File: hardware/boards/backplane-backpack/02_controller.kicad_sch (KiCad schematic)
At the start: 12 parts, among them J10 GND/+3V3/SWDIO/SWCLK/NRST (TB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, U1 STM32C092FCP6

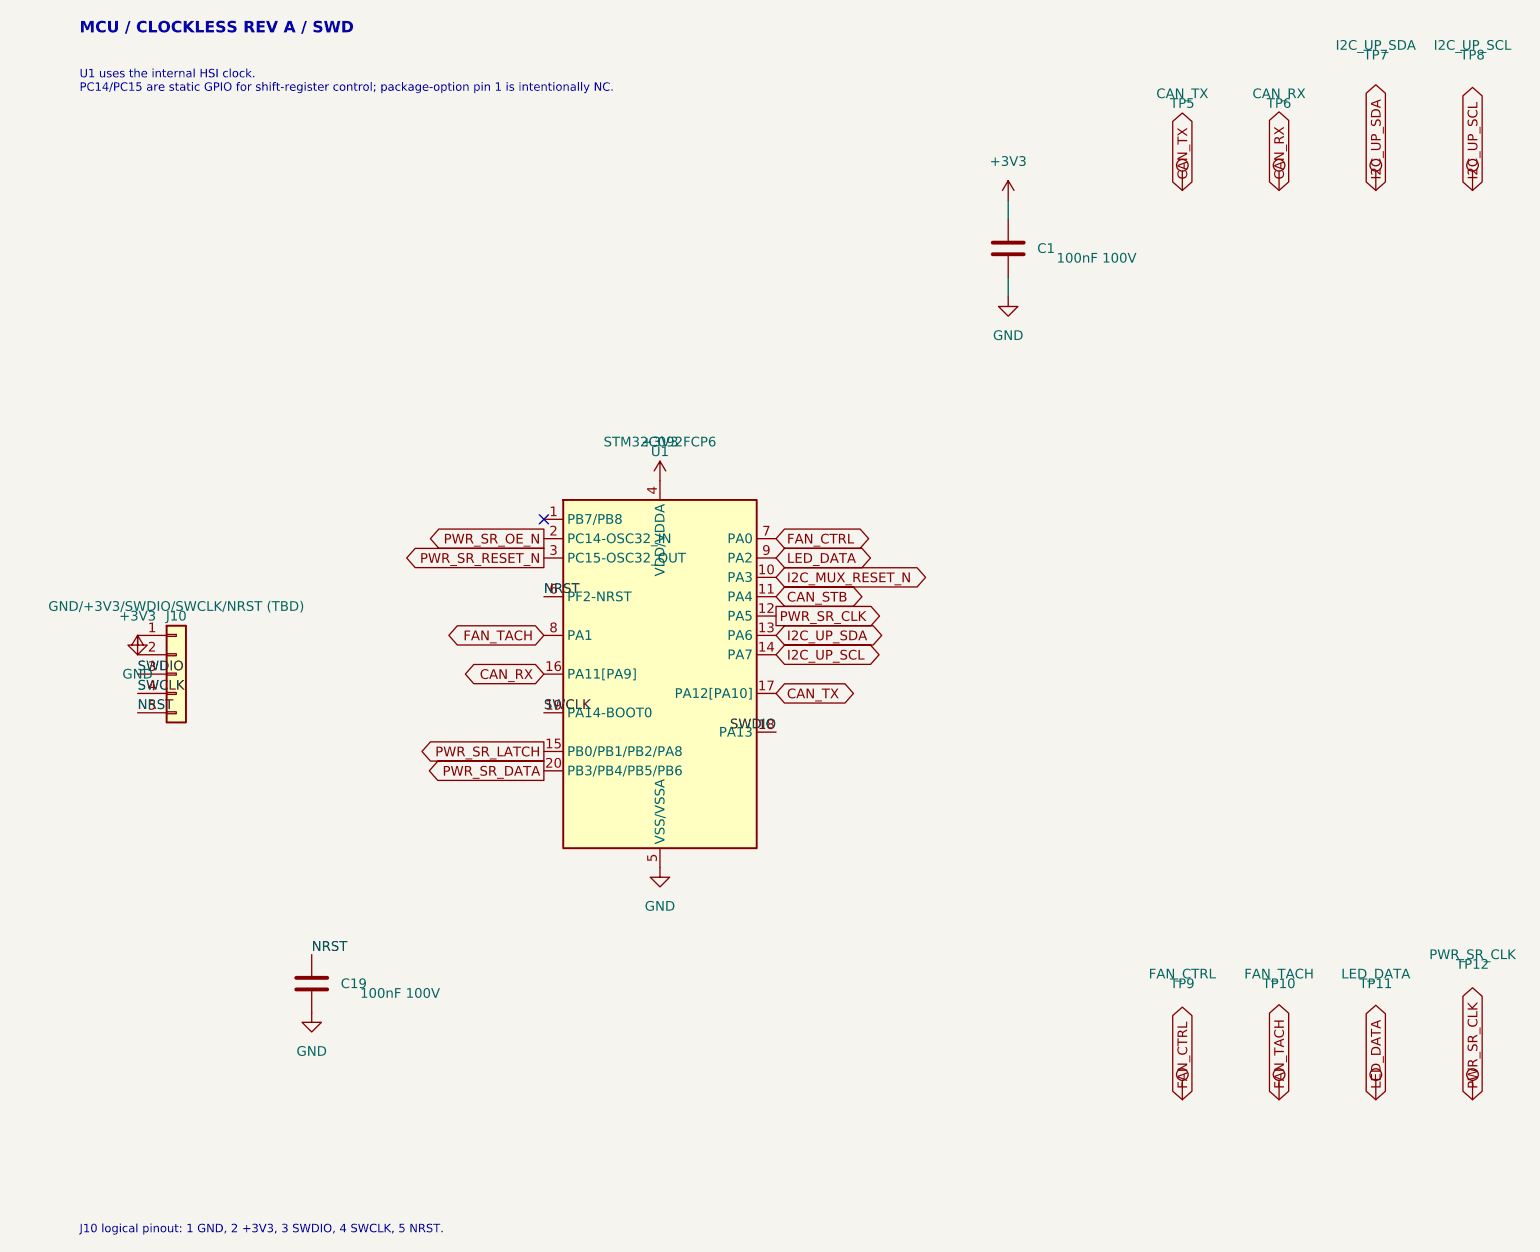
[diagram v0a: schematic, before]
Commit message: chore: checkpoint current board layout
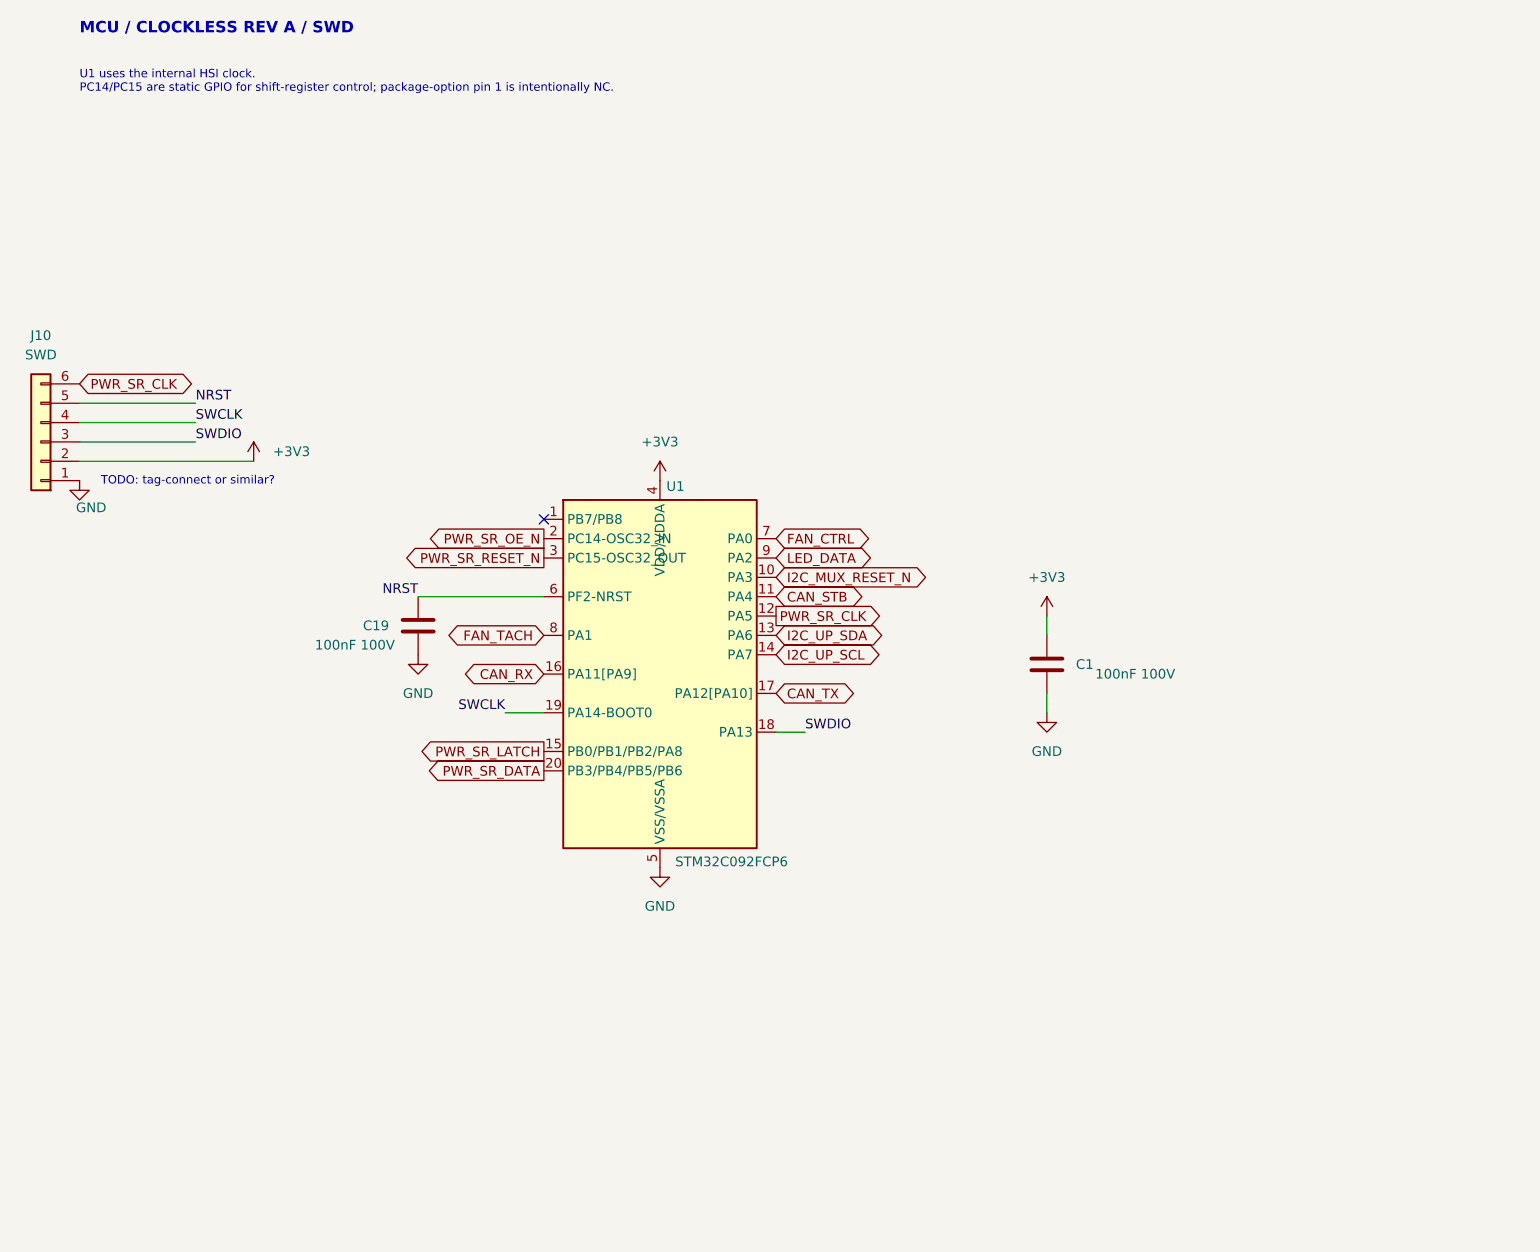
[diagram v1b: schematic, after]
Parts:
- removed J10: GND/+3V3/SWDIO/SWCLK/NRST (TBD), symbol Connector_Generic:Conn_01x05
- removed TP10: FAN_TACH, TestPoint:TestPoint_Pad_D1.5mm, symbol Connector:TestPoint
- removed TP11: LED_DATA, TestPoint:TestPoint_Pad_D1.5mm, symbol Connector:TestPoint
- removed TP12: PWR_SR_CLK, TestPoint:TestPoint_Pad_D1.5mm, symbol Connector:TestPoint
- removed TP5: CAN_TX, TestPoint:TestPoint_Pad_D1.5mm, symbol Connector:TestPoint
- removed TP6: CAN_RX, TestPoint:TestPoint_Pad_D1.5mm, symbol Connector:TestPoint
- removed TP7: I2C_UP_SDA, TestPoint:TestPoint_Pad_D1.5mm, symbol Connector:TestPoint
- removed TP8: I2C_UP_SCL, TestPoint:TestPoint_Pad_D1.5mm, symbol Connector:TestPoint
- removed TP9: FAN_CTRL, TestPoint:TestPoint_Pad_D1.5mm, symbol Connector:TestPoint
- added J10: SWD, symbol Connector_Generic:Conn_01x06
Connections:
- net +3V3: now also J10.2 (Pin_2)
- net GND: now also J10.1 (Pin_1)
- net NRST: now also J10.5 (Pin_5)
- net PWR_SR_CLK: now also J10.6 (Pin_6)
- net SWCLK: now also J10.4 (Pin_4)
- net SWDIO: now also J10.3 (Pin_3)
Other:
- note added: "TODO: tag-connect or similar?"
- note removed: "J10 logical pinout: 1 GND, 2 +3V3, 3 SWDIO, 4 SWCLK, 5 NRST."
- moved on the sheet: C1, C19
